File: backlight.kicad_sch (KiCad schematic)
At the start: 32 parts

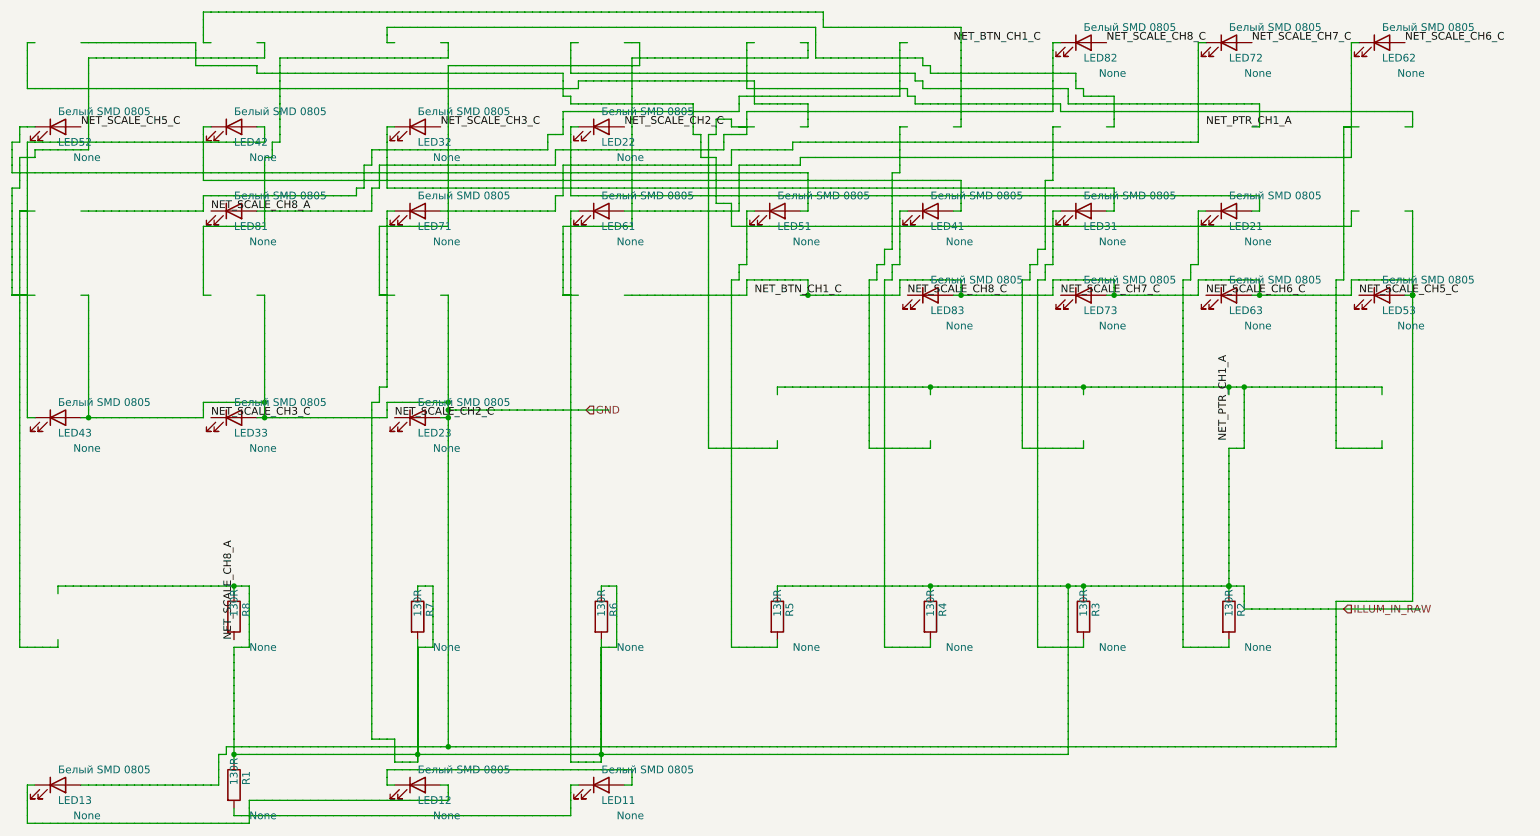
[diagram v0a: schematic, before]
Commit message: fix writer
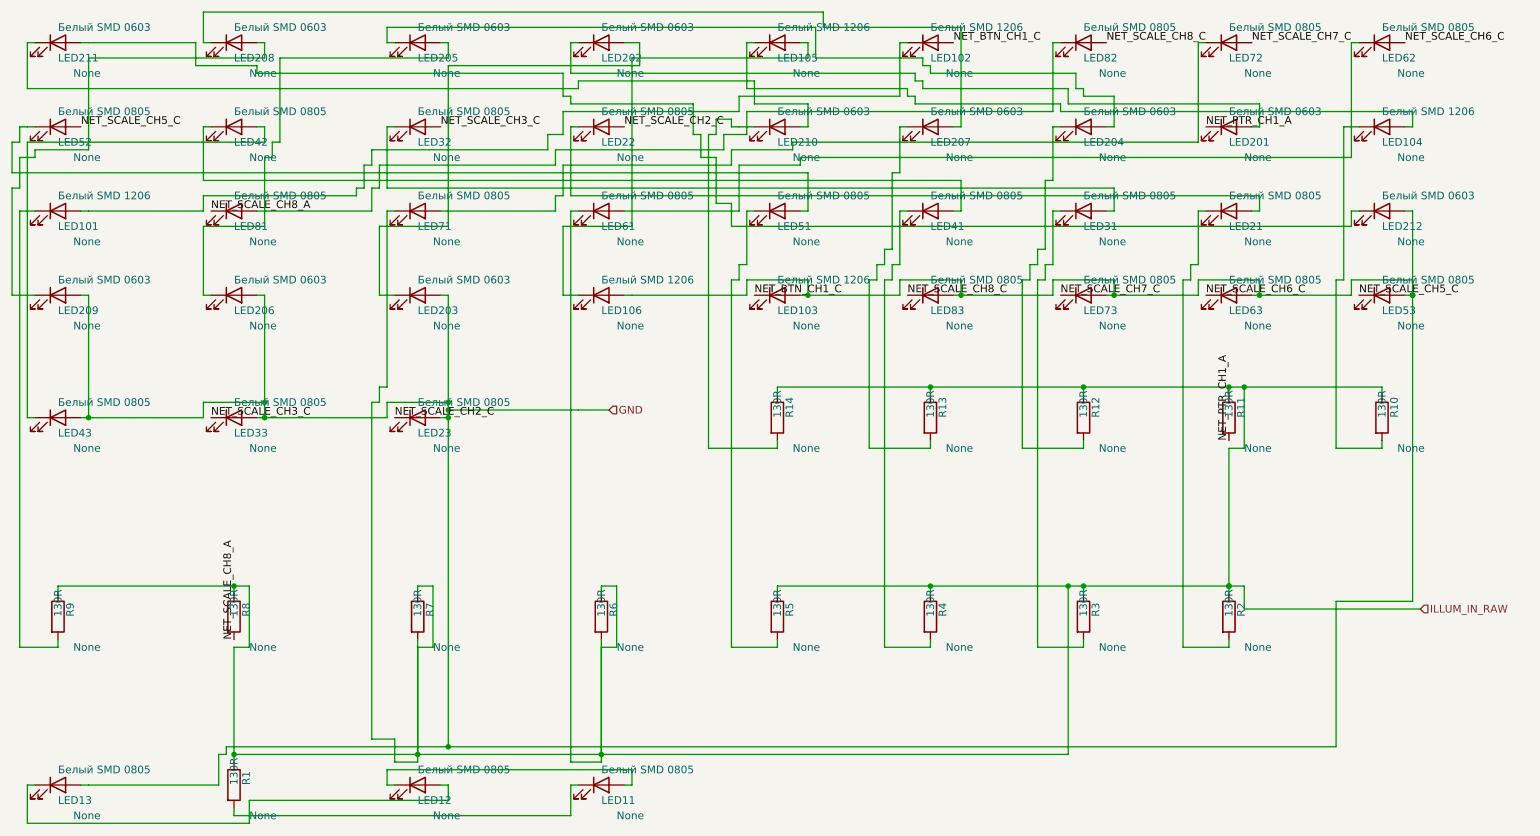
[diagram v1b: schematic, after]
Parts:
- added LED101, LED102, LED103, LED104, LED105, LED106: Белый SMD 1206, symbol Device:LED
- added LED201, LED202, LED203, LED204, LED205, LED206, LED207, LED208, LED209, LED210, LED211, LED212: Белый SMD 0603, symbol Device:LED
- added R10, R11, R12, R13, R14, R9: 130R, symbol Device:R
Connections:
- net GND: now also LED103.2 (A), LED106.2 (A), LED203.2 (A), LED206.2 (A), LED209.2 (A), LED212.2 (A); no longer LED21.1 (K), LED21.2 (A), LED22.1 (K), LED31.1 (K), LED31.2 (A), LED32.1 (K), LED41.1 (K), LED41.2 (A), LED42.1 (K), LED42.2 (A), LED43.1 (K), LED51.1 (K), LED51.2 (A), LED52.1 (K), LED61.1 (K), LED61.2 (A), LED62.1 (K), LED71.1 (K), LED71.2 (A), LED72.1 (K), LED81.2 (A), LED82.1 (K), R1.1, R2.1, R2.2, R3.1, R3.2, R4.1, R4.2, R5.1, R5.2, R6.1, R6.2, R7.1, R7.2, R8.1
- net NET_BTN_CH1_C: now also LED102.2 (A), LED103.1 (K)
- net NET_PTR_CH1_A: now also LED201.1 (K), R11.2
- net at LED11.1 (K), R1.2: no longer LED12.2 (A), LED13.1 (K)
- new net: LED101.1 (K), R9.2
- new net: LED204.1 (K), R12.2
- new net: LED204.2 (A), LED205.1 (K)
- new net: LED207.1 (K), R13.2
- new net: LED207.2 (A), LED208.1 (K)
- new net: LED205.2 (A), LED206.1 (K)
- new net: LED21.1 (K), R2.2
- new net: LED21.2 (A), LED22.1 (K)
- new net: LED81.2 (A), LED82.1 (K)
- new net: LED51.1 (K), R5.2
- new net: LED208.2 (A), LED209.1 (K)
- new net: LED202.2 (A), LED203.1 (K)
- new net: LED101.2 (A), LED102.1 (K)
- new net: LED41.2 (A), LED42.1 (K)
- new net: LED42.2 (A), LED43.1 (K)
- new net: LED201.2 (A), LED202.1 (K)
- new net: LED104.1 (K), R10.2
- new net: LED104.2 (A), LED105.1 (K)
- new net: LED41.1 (K), R4.2
- new net: LED105.2 (A), LED106.1 (K)
- new net: LED71.2 (A), LED72.1 (K)
- new net: LED31.1 (K), R3.2
- new net: LED31.2 (A), LED32.1 (K)
- new net: LED210.1 (K), R14.2
- new net: LED61.2 (A), LED62.1 (K)
- new net: LED51.2 (A), LED52.1 (K)
- new net: LED210.2 (A), LED211.1 (K)
- new net: LED211.2 (A), LED212.1 (K)
- new net: LED12.2 (A), LED13.1 (K)
- new net ILLUM_IN_RAW: LED61.1 (K), LED71.1 (K), R1.1, R10.1, R11.1, R12.1, R13.1, R14.1, R2.1, R3.1, R4.1, R5.1, R6.1, R6.2, R7.1, R7.2, R8.1, R9.1
